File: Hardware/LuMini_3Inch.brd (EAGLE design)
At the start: 76.2 x 76.2 mm, 88 parts, among them J1 DOUBLE_LED_PAD, J2 DOUBLE_LED_PAD, J3 DOUBLE_LED_PAD

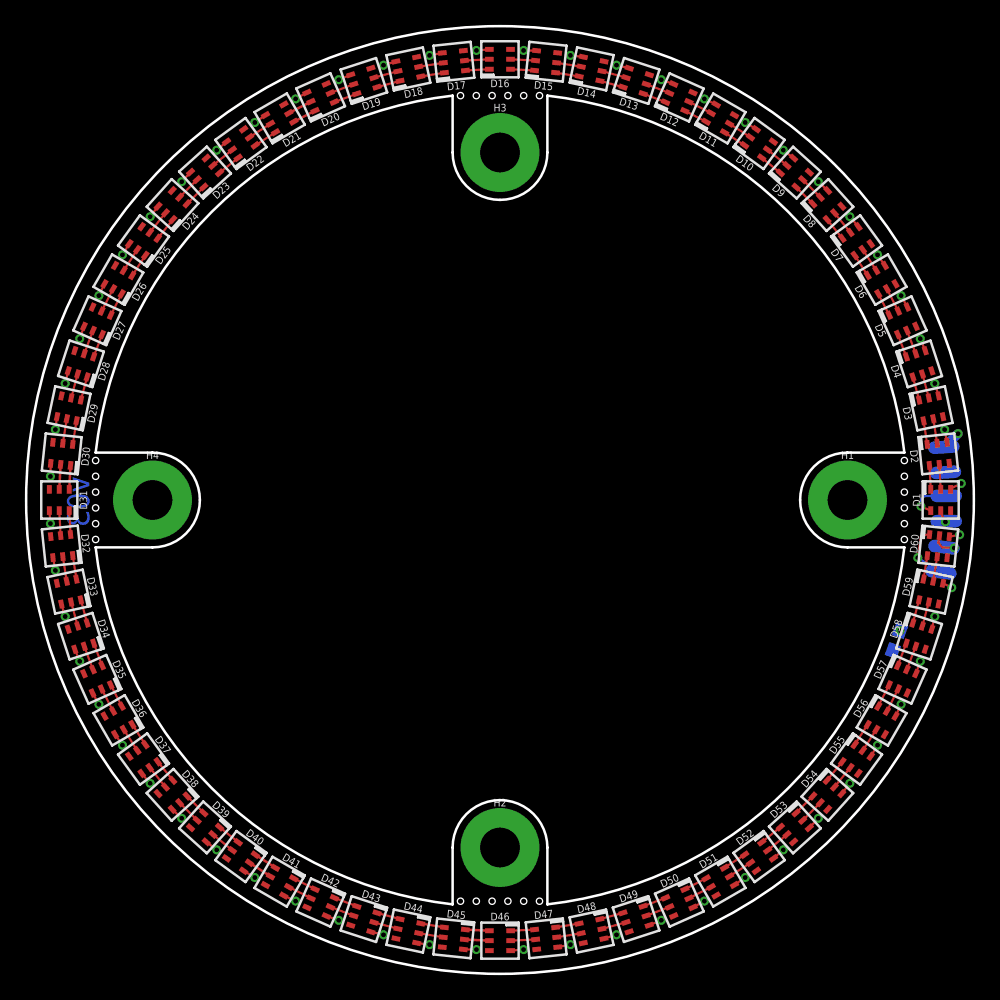
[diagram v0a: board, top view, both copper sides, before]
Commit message: post checklist
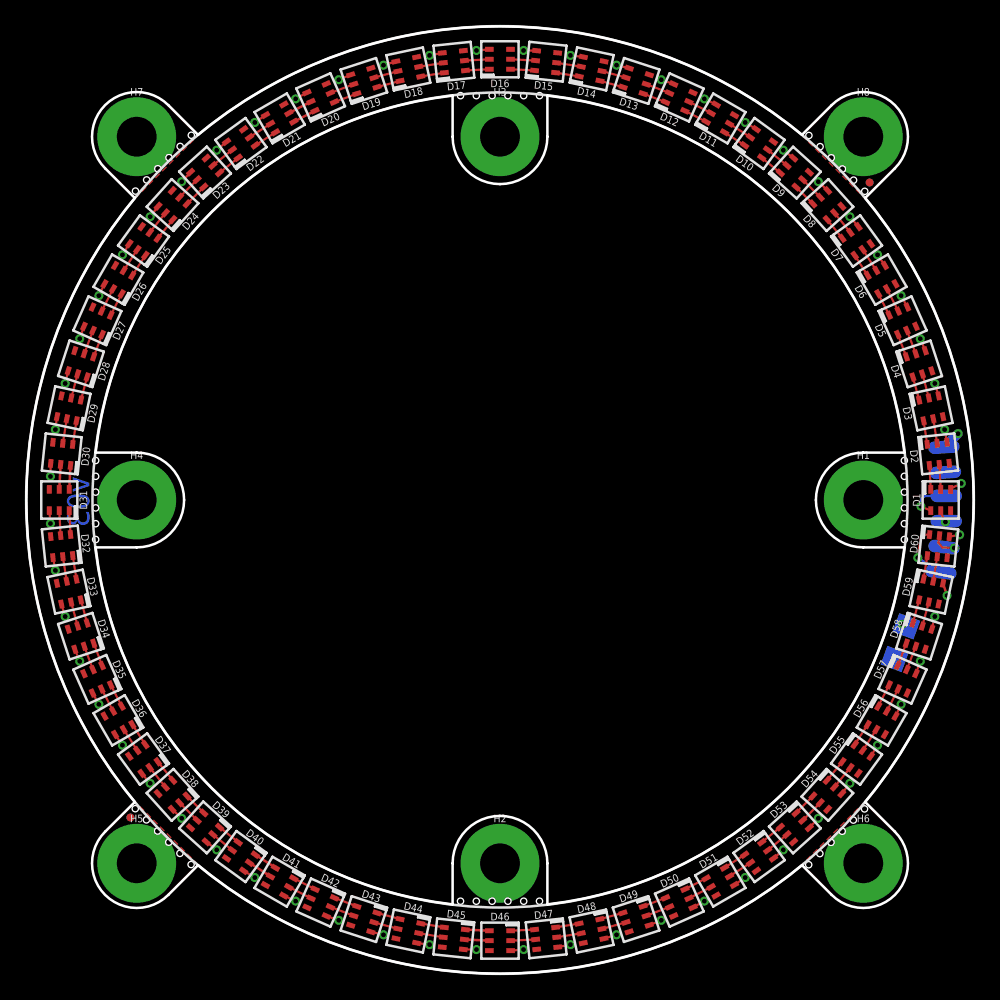
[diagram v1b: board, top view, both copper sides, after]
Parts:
- added FD1, FD2, FD3, FD4: FIDUCIALUFIDUCIAL, SparkFun-Aesthetics:FIDUCIAL-MICRO
- added H5, H6, H7, H8: STANDOFF_ELECTRICALSTANDOFF-ELECTRICAL-NOTHERMALS, SparkFun-Hardware:STANDOFF-ELECTRICAL-NOTHERMALS
- added U$18: (no value), SparkFun-Aesthetics:ORDERING_INSTRUCTIONS
- C1: value 4.7uF -> DNP; device SparkFun-Capacitors:0603 -> SparkFun-Capacitors:1206
- U$1: device buzzard_labels (2):LUMINI0 -> buzzard_labels (8):LUMINI_3#2
- moved H2 1.27 mm to (38.1, 8.89)
- moved H4 1.27 mm to (8.89, 38.1)
- moved H1 1.27 mm to (67.3, 38.1)
- moved H3 1.27 mm to (38.1, 67.3)
- moved U$1 0.89 mm to (34.0, 1.08)
- moved C1 0.36 mm to (70.3, 26.6)
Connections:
- net GND: now also H5.P1, H6.P1, H7.P1, H8.P1
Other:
- outline, holes or cut-outs redrawn
- board text added: "Black PCB 2 Oz. Cu"

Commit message: cleaning up schematic
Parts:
- H1, H2, H3, H4, H5, H6, H7, H8: value STANDOFF_ELECTRICALSTANDOFF-ELECTRICAL-NOTHERMALS -> STANDOFF_ELECTRICAL-NOTHERMALS
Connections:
- net N$122 renamed CO
- net N$123 renamed DO
- net N$2 renamed CI
- net N$3 renamed DI
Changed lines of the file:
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@@
 <attribute name="REV" value="" x="14.605" y="-8.255" size="1.778" layer="27" display="off"/>
 </element>
-<element name="H1" library="SparkFun-Hardware" package="STANDOFF-ELECTRICAL-NOTHERMALS" value="STANDOFF_ELECTRICALSTANDOFF-ELECTRICAL-NOTHERMALS" x="67.31" y="38.1"/>
-<element name="H2" library="SparkFun-Hardware" package="STANDOFF-ELECTRICAL-NOTHERMALS" value="STANDOFF_ELECTRICALSTANDOFF-ELECTRICAL-NOTHERMALS" x="38.1" y="8.89"/>
-<element name="H3" library="SparkFun-Hardware" package="STANDOFF-ELECTRICAL-NOTHERMALS" value="STANDOFF_ELECTRICALSTANDOFF-ELECTRICAL-NOTHERMALS" x="38.1" y="67.31"/>
-<element name="H4" library="SparkFun-Hardware" package="STANDOFF-ELECTRICAL-NOTHERMALS" value="STANDOFF_ELECTRICALSTANDOFF-ELECTRICAL-NOTHERMALS" x="8.89" y="38.1"/>
+<element name="H1" library="SparkFun-Hardware" package="STANDOFF-ELECTRICAL-NOTHERMALS" value="STANDOFF_ELECTRICAL-NOTHERMALS" x="67.31" y="38.1"/>
+<element name="H2" library="SparkFun-Hardware" package="STANDOFF-ELECTRICAL-NOTHERMALS" value="STANDOFF_ELECTRICAL-NOTHERMALS" x="38.1" y="8.89"/>
+<element name="H3" library="SparkFun-Hardware" package="STANDOFF-ELECTRICAL-NOTHERMALS" value="STANDOFF_ELECTRICAL-NOTHERMALS" x="38.1" y="67.31"/>
+<element name="H4" library="SparkFun-Hardware" package="STANDOFF-ELECTRICAL-NOTHERMALS" value="STANDOFF_ELECTRICAL-NOTHERMALS" x="8.89" y="38.1"/>
 <element name="C1" library="SparkFun-Capacitors" package="1206" value="DNP" x="70.2945" y="26.6319" rot="MR110">
 <attribute name="PROD_ID" value="CAP-10300" x="70.2945" y="26.6319" size="1.778" layer="28" rot="MR110" display="off"/>
@@
 <element name="U$16" library="buzzard_labels (5)" package="5013" value="" x="54.1528" y="6.4897" rot="MR150"/>
 <element name="U$17" library="buzzard_labels (5)" package="5514" value="" x="67.9704" y="18.9611" rot="MR120"/>
-<element name="H5" library="SparkFun-Hardware" package="STANDOFF-ELECTRICAL-NOTHERMALS" value="STANDOFF_ELECTRICALSTANDOFF-ELECTRICAL-NOTHERMALS" x="8.89" y="8.89"/>
-<element name="H6" library="SparkFun-Hardware" package="STANDOFF-ELECTRICAL-NOTHERMALS" value="STANDOFF_ELECTRICALSTANDOFF-ELECTRICAL-NOTHERMALS" x="67.31" y="8.89"/>
-<element name="H7" library="SparkFun-Hardware" package="STANDOFF-ELECTRICAL-NOTHERMALS" value="STANDOFF_ELECTRICALSTANDOFF-ELECTRICAL-NOTHERMALS" x="8.89" y="67.31"/>
-<element name="H8" library="SparkFun-Hardware" package="STANDOFF-ELECTRICAL-NOTHERMALS" value="STANDOFF_ELECTRICALSTANDOFF-ELECTRICAL-NOTHERMALS" x="67.31" y="67.31"/>
+<element name="H5" library="SparkFun-Hardware" package="STANDOFF-ELECTRICAL-NOTHERMALS" value="STANDOFF_ELECTRICAL-NOTHERMALS" x="8.89" y="8.89"/>
+<element name="H6" library="SparkFun-Hardware" package="STANDOFF-ELECTRICAL-NOTHERMALS" value="STANDOFF_ELECTRICAL-NOTHERMALS" x="67.31" y="8.89"/>
+<element name="H7" library="SparkFun-Hardware" package="STANDOFF-ELECTRICAL-NOTHERMALS" value="STANDOFF_ELECTRICAL-NOTHERMALS" x="8.89" y="67.31"/>
+<element name="H8" library="SparkFun-Hardware" package="STANDOFF-ELECTRICAL-NOTHERMALS" value="STANDOFF_ELECTRICAL-NOTHERMALS" x="67.31" y="67.31"/>
 <element name="FD1" library="SparkFun-Aesthetics" package="FIDUCIAL-MICRO" value="FIDUCIALUFIDUCIAL" x="8.382" y="12.573"/>
 <element name="FD2" library="SparkFun-Aesthetics" package="FIDUCIAL-MICRO" value="FIDUCIALUFIDUCIAL" x="8.382" y="12.573" rot="MR90"/>
@@
 <wire x1="74.041" y1="30.4165" x2="73.72008125" y2="31.401634375" width="0.2032" layer="1"/>
 </signal>
-<signal name="N$2">
+<signal name="CI">
 <contactref element="D1" pad="CKI"/>
 <contactref element="J2" pad="P$2"/>
@@
 <wire x1="73.9775" y1="36.3982" x2="73.914" y2="36.3347" width="0.1778" layer="16"/>
 </signal>
-<signal name="N$3">
+<signal name="DI">
 <contactref element="D1" pad="SDI"/>
 <contactref element="J2" pad="P$1"/>
@@
 <wire x1="69.2082" y1="21.117078125" x2="70.121490625" y2="22.914065625" width="0.1778" layer="1"/>
 </signal>
-<signal name="N$122">
+<signal name="CO">
 <contactref element="D60" pad="CKO"/>
 <contactref element="J3" pad="P$2"/>
@@
 <wire x1="73.3425" y1="34.671" x2="73.66" y2="34.29" width="0.1778" layer="1"/>
 </signal>
-<signal name="N$123">
+<signal name="DO">
 <contactref element="D60" pad="SDO"/>
 <contactref element="J3" pad="P$1"/>

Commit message: fixing library issue
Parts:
- J1, J2, J3: value DOUBLE_LED_PAD -> SOLDER_PAD_2; device Andy:DOUBLELEDPAD -> SparkFun-Connectors:SOLDER_PAD_2
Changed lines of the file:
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@@
 <attribute name="PROD_ID" value="DIO-13883" x="37.41715" y="64.91578125" size="1.778" layer="27" rot="R204" display="off"/>
 </element>
-<element name="J1" library="Andy" package="DOUBLELEDPAD" value="DOUBLE_LED_PAD" x="73.8505" y="41.3385" rot="MR266.4"/>
-<element name="J2" library="Andy" package="DOUBLELEDPAD" value="DOUBLE_LED_PAD" x="73.9775" y="37.4142" rot="MR270"/>
+<element name="J1" library="SparkFun-Connectors" package="SOLDER_PAD_2" value="SOLDER_PAD_2" x="73.8505" y="41.3385" rot="MR266.4"/>
+<element name="J2" library="SparkFun-Connectors" package="SOLDER_PAD_2" value="SOLDER_PAD_2" x="73.9775" y="37.4142" rot="MR270"/>
 <element name="U$1" library="buzzard_labels (8)" package="LUMINI_3#2" value="" x="34.036" y="1.0795" rot="MR180"/>
 <element name="U$4" library="buzzard_labels (25)" package="5V6" value="" x="71.6915" y="41.529" rot="MR266.4"/>
@@
 <attribute name="PROD_ID" value="DIO-13883" x="35.38531875" y="-72.599775" size="1.778" layer="27" rot="R84" display="off"/>
 </element>
-<element name="J3" library="Andy" package="DOUBLELEDPAD" value="DOUBLE_LED_PAD" x="73.6727" y="33.2994" rot="MR97"/>
+<element name="J3" library="SparkFun-Connectors" package="SOLDER_PAD_2" value="SOLDER_PAD_2" x="73.6727" y="33.2994" rot="MR97"/>
 <element name="U$2" library="buzzard_labels (3)" package="60_APA102_LEDS0" value="" x="31.5595" y="4.0005" rot="MR180"/>
 <element name="FRAME1" library="SparkFun-Aesthetics" package="CREATIVE_COMMONS" value="FRAME-LEDGER" x="14.605" y="-8.255">
